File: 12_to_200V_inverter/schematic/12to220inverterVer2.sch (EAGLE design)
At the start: 37 parts, among them IC10 MC34063, T11 BC857, T15 IRL5602S, T16 BC847, T17 IRF830, X1 +12V_INPUT, X2 200VDC_OUTPUT, X3 TURN_ON

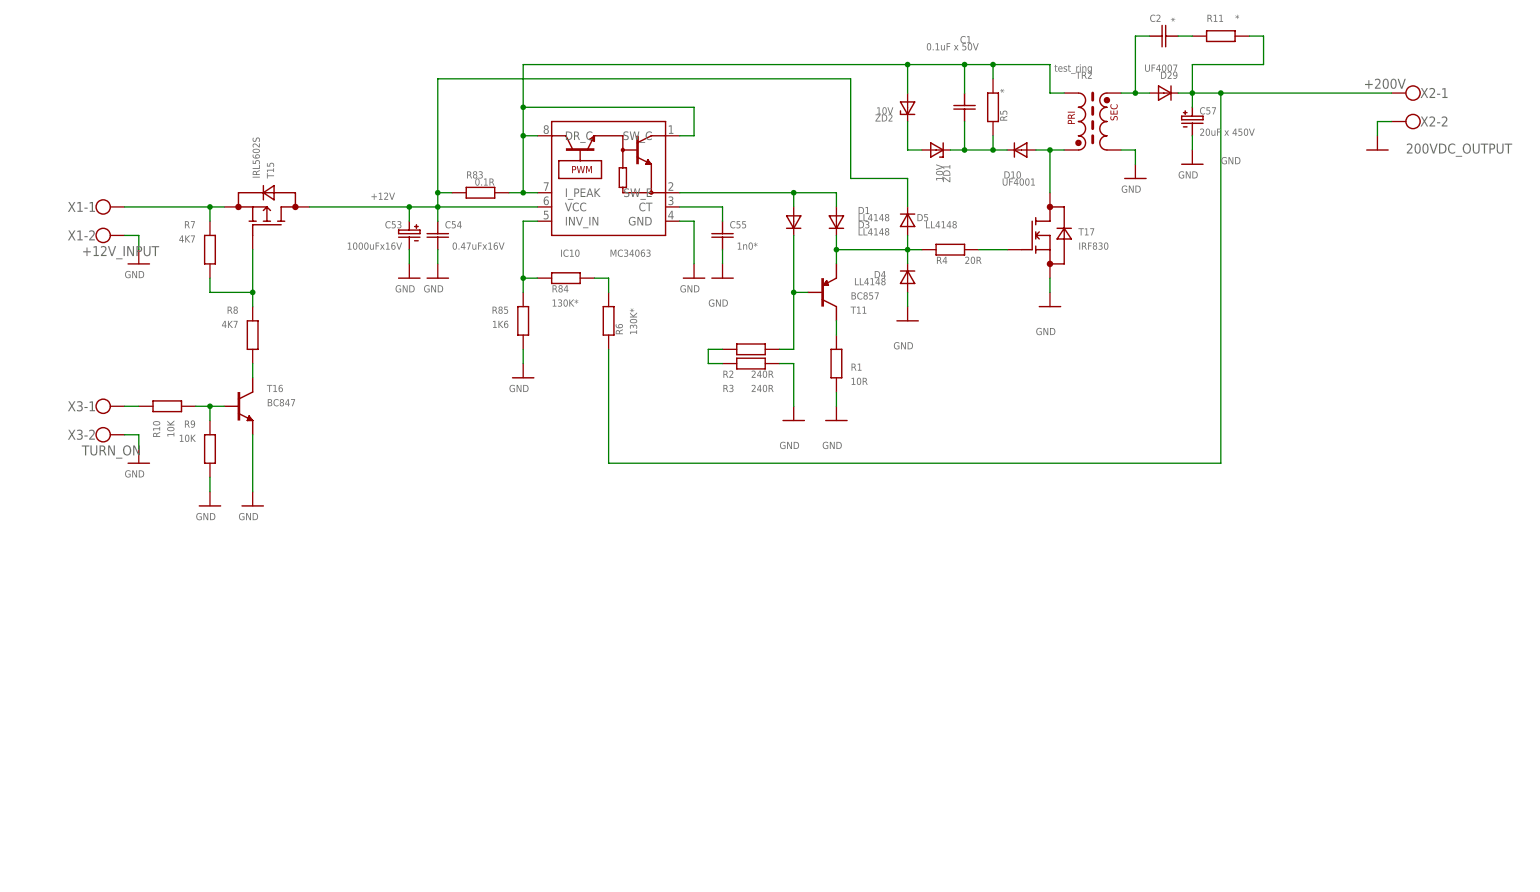
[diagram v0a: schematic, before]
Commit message: 12 to 200V converter v2. Forward 2 conversion.
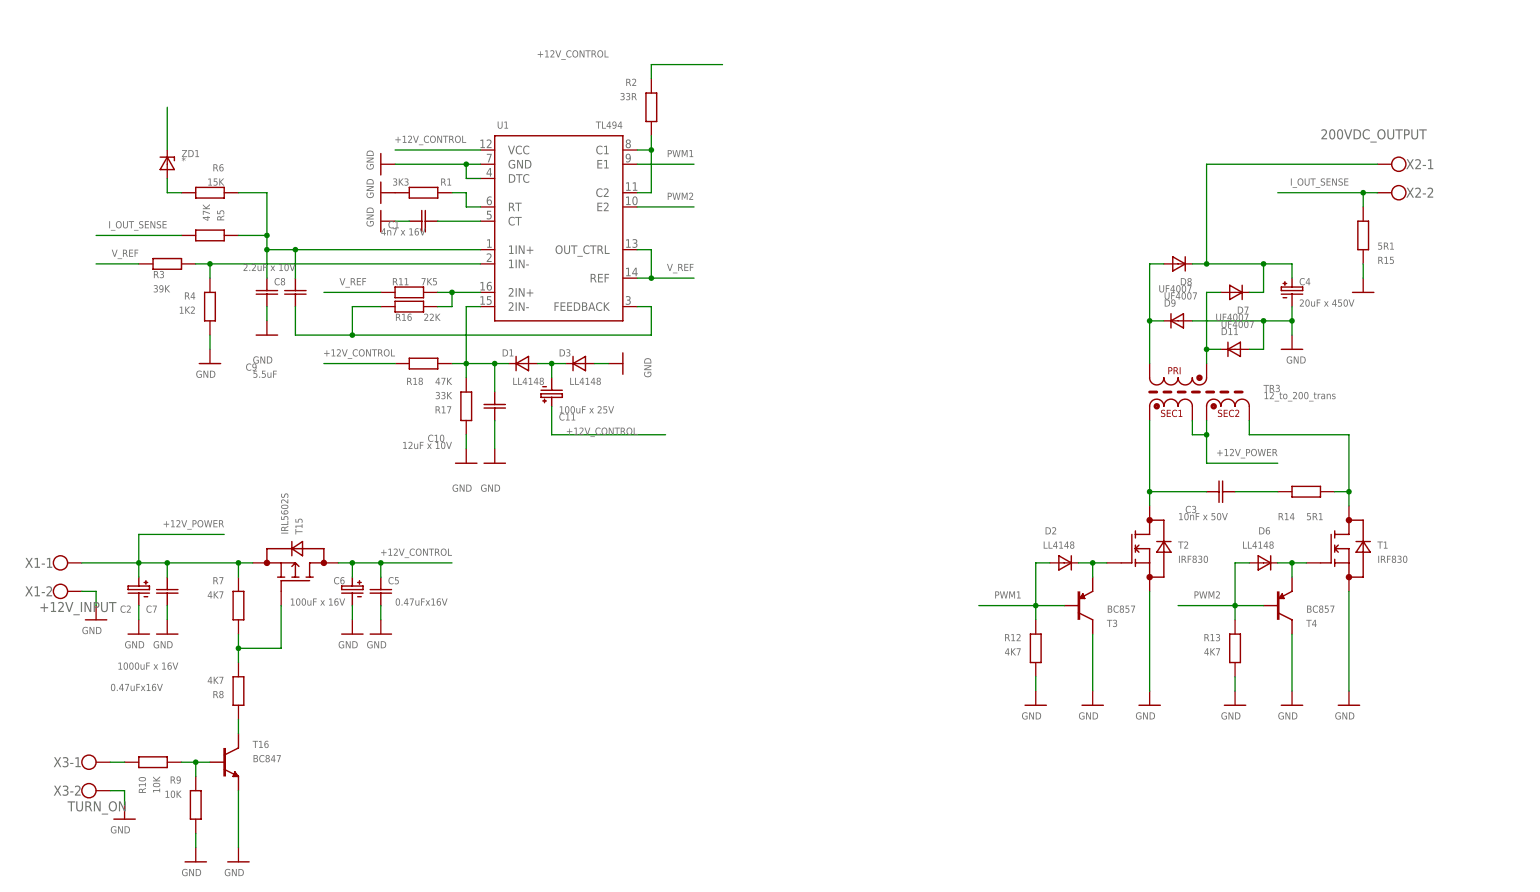
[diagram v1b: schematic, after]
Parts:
- removed C53: 1000uFx16V, __MyCommonLib1:CE16MM
- removed C54: 0.47uFx16V, __MyCommonLib1:CSMD_1206
- removed C55: 1n0*, __MyCommonLib1:CSMD_0805
- removed C57: 20uF x 450V, __MyCommonLib1:CE16MM
- removed D10: UF4001, __MyCommonLib1:1N4001DO-41_15MM
- removed D29: UF4007, __MyCommonLib1:1N4001DO-41_10MM
- removed D4, D5: LL4148, __MyCommonLib1:LL4147SOD-80
- removed IC10: MC34063, __MyCommonLib1:MC34063(DIP8)
- removed R83: 0.1R, __MyCommonLib1:RSMD_2512
- removed R84: 130K*, __MyCommonLib1:RSMD_1206
- removed R85: 1K6, __MyCommonLib1:RSMD_0805
- removed T11: BC857, __MyCommonLib1:BC857SOT23_SMALL_PADS
- removed T17: IRF830, __MyCommonLib1:IRF830TO-220
- removed TR2: test_ring, __MyCommonLib1:TRANS_2WIND(RING_25X10)
- removed ZD2: 10V, __MyCommonLib1:ZENNER(SOD_80)
- added C10: 12uF x 10V, __MyCommonLib1:CSMD_0805
- added C11: 100uF x 25V, __MyCommonLib1:CE5.2MM
- added C3: 10nF x 50V, __MyCommonLib1:CSMD_1206
- added C4: 20uF x 450V, __MyCommonLib1:CE16MM
- added C5, C7: 0.47uFx16V, __MyCommonLib1:CSMD_1206
- added C6: 100uF x 16V, __MyCommonLib1:CE8.2MM
- added C8: 2.2uF x 10V, __MyCommonLib1:CSMD_0805
- added C9: 5.5uF, __MyCommonLib1:CSMD_0805
- added D11, D7, D8, D9: UF4007, __MyCommonLib1:1N4001DO-41_10MM
- added D2, D6: LL4148, __MyCommonLib1:LL4147SOD-80
- added R12, R13: 4K7, __MyCommonLib1:RSMD_0805
- added R14, R15: 5R1, __MyCommonLib1:RSMD_1206
- added R16: 22K, __MyCommonLib1:RSMD_0805
- added R17: 33K, __MyCommonLib1:RSMD_0805
- added R18: 47K, __MyCommonLib1:RSMD_0805
- added T1, T2: IRF830, __MyCommonLib1:IRF830TO-220
- added T3, T4: BC857, __MyCommonLib1:BC857SOT23_SMALL_PADS
- added TR3: 12_to_200_trans, __MyCommonLib1:TRANS_38X30MM
- added U1: TL494, __MyCommonLib1:TL494(SOIC-16)
- C1: value 0.1uF x 50V -> 4n7 x 16V; device __MyCommonLib1:CSMD_1206 -> __MyCommonLib1:CSMD_0805
- C2: value * -> 1000uF x 16V; device __MyCommonLib1:CSMD_1206 -> __MyCommonLib1:CE16MM
- R1: value 10R -> 3K3; device __MyCommonLib1:RSMD_1206_BIG_GAP -> __MyCommonLib1:RSMD_0805
- R11: value * -> 7K5; device __MyCommonLib1:RSMD_1206 -> __MyCommonLib1:RSMD_0805
- R2: value 240R -> 33R; device __MyCommonLib1:RSMD_1206_BIG_GAP -> __MyCommonLib1:RSMD_0805
- R3: value 240R -> 39K; device __MyCommonLib1:RSMD_1206_BIG_GAP -> __MyCommonLib1:RSMD_0805
- R4: value 20R -> 1K2
- R5: value * -> 47K; device __MyCommonLib1:RSMD_1206 -> __MyCommonLib1:RSMD_0805
- R6: value 130K* -> 15K; device __MyCommonLib1:RSMD_1206 -> __MyCommonLib1:RSMD_0805
- ZD1: value 10V -> *
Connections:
- removed net +12V: C53.PLUS, C54.PIN1, D5.CATHODE, IC10.VCC, R83.PIN0, T15.DRAIN
- removed net +200V: C57.PLUS, D29.CATHODE, R11.PIN0, R6.PIN0, X2-1.KL
- removed net N$1: D10.ANODE, T17.DRAIN, TR2.PRI_START
- removed net N$10: C1.PIN1, IC10.DR_C, IC10.I_PEAK, IC10.SW_C, R5.PIN1, R83.PIN1, TR2.PRI_END, ZD2.ANODE
- removed net N$11: C2.PIN1, D29.ANODE, TR2.SEC_START
- removed net N$135: C55.PIN1, IC10.CT
- removed net N$139: IC10.INV_IN, R84.PIN0, R85.PIN1
- new net +12V_CONTROL: C11.PLUS, C5.PIN1, C6.PLUS, R18.PIN1, R2.PIN1, T15.DRAIN, U1.VCC
- new net +12V_POWER: C2.PLUS, C7.PIN1, R7.PIN1, T15.SOURCE, TR3.SEC1_END, TR3.SEC2_START, X1-1.KL
- new net I_OUT_SENSE: R15.PIN0, R5.PIN1, X2-2.KL
- new net N$19: D2.CATHODE, T2.GATE, T3.E
- new net N$20: D11.CATHODE, D7.ANODE, TR3.PRI_START
- new net N$21: D6.CATHODE, T1.GATE, T4.E
- new net N$23: D8.ANODE, D9.CATHODE, TR3.PRI_END
- new net N$24: C3.PIN1, T2.DRAIN, TR3.SEC1_START
- new net N$25: R14.PIN0, T1.DRAIN, TR3.SEC2_END
- new net N$26: C3.PIN0, R14.PIN1
- new net N$28: C4.PLUS, D7.CATHODE, D8.CATHODE, X2-1.KL
- new net PWM1: D2.ANODE, R12.PIN1, T3.B, U1.E1
- new net PWM2: D6.ANODE, R13.PIN1, T4.B, U1.E2
- new net V_REF: R11.PIN1, R3.PIN1, U1.OUT_CTRL, U1.REF
- net GND: now also C1.PIN1, C10.PIN0, C2.MINUS, C4.MINUS, C5.PIN0, C6.MINUS, C7.PIN0, C9.PIN0, D11.ANODE, D3.ANODE, D9.ANODE, R1.PIN0, R12.PIN0, R13.PIN0, R15.PIN1, R17.PIN1, R4.PIN1, T1.SOURCE, T2.SOURCE, T3.C, T4.C, U1.DTC, U1.GND; no longer C53.MINUS, C54.PIN0, C55.PIN0, C57.MINUS, D4.ANODE, IC10.GND, R1.PIN1, R3.PIN1, R85.PIN0, T17.SOURCE, TR2.SEC_END, X2-2.KL
- net N$12: now also R11.PIN0, R16.PIN0, U1.2IN+; no longer ZD1.ANODE, ZD2.CATHODE
- net N$13: now also C11.MINUS, D1.ANODE, D3.CATHODE; no longer R7.PIN1, T15.SOURCE, X1-1.KL
- net N$18: now also C10.PIN1, D1.CATHODE, R17.PIN0, R18.PIN0, U1.2IN-; no longer C2.PIN0, R11.PIN1
- net N$2: now also C1.PIN0, U1.CT; no longer R1.PIN0, T11.C
- net N$3: now also R1.PIN1, U1.RT; no longer R6.PIN1, R84.PIN1
- net N$4: now also U1.C1, U1.C2; no longer D3.CATHODE, T11.B
- net N$5: now also R4.PIN0, U1.1IN-; no longer R2.PIN1
- net N$6: now also C8.PIN0, R16.PIN1, U1.FEEDBACK; no longer D1.ANODE, D3.ANODE, IC10.SW_E
- net N$7: now also C8.PIN1, C9.PIN1, R5.PIN0, R6.PIN0, U1.1IN+; no longer D1.CATHODE, D4.CATHODE, D5.ANODE, R4.PIN0, T11.E
- net N$8: now also R6.PIN1, ZD1.ANODE; no longer R4.PIN1, T17.GATE
- net N$9: no longer C1.PIN0, D10.CATHODE, R5.PIN0
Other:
- moved on the sheet: C1, D1, D3, R1, R10, R11, R2, R3, R4, R5, R6, R7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
